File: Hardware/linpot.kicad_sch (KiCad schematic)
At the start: 7 parts, among them U7 Opamp_Dual

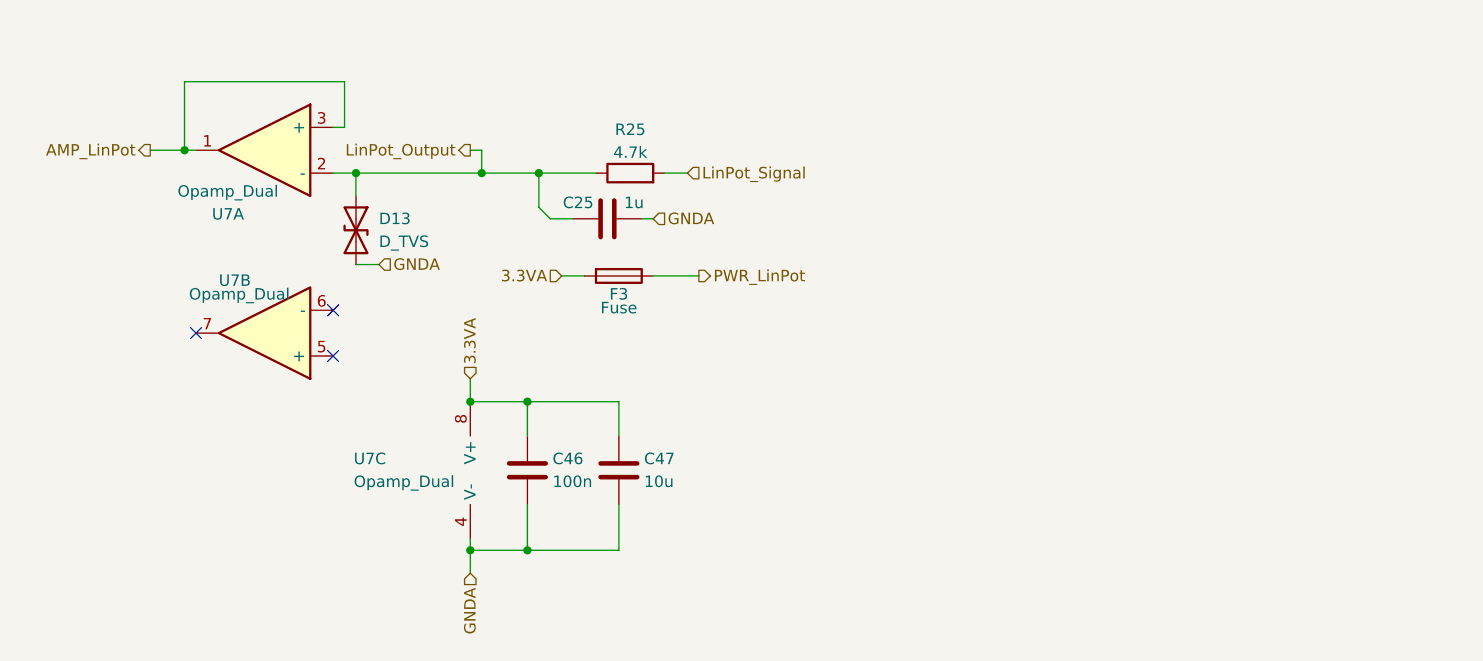
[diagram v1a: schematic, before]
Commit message: made review changes
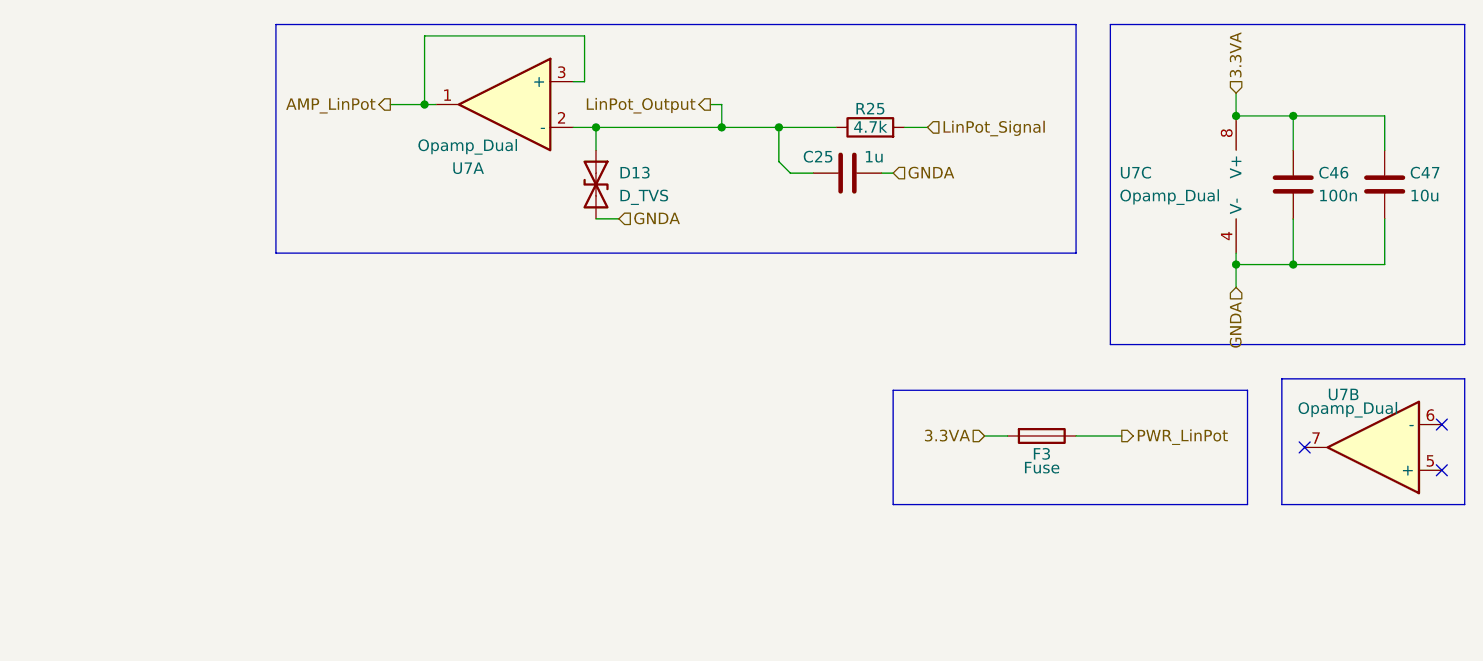
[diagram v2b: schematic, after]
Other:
- moved on the sheet: C25, C46, C47, D13, F3, R25, U7A, U7B, U7C
